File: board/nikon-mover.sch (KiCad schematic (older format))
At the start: 18 parts, among them IC1 ATMEGA8-P, J1 USB, P1 CONN_5, P2 CONN_5, P3 CONN_1, P4 CONN_1, U1 ULN2803, X1 16MHz

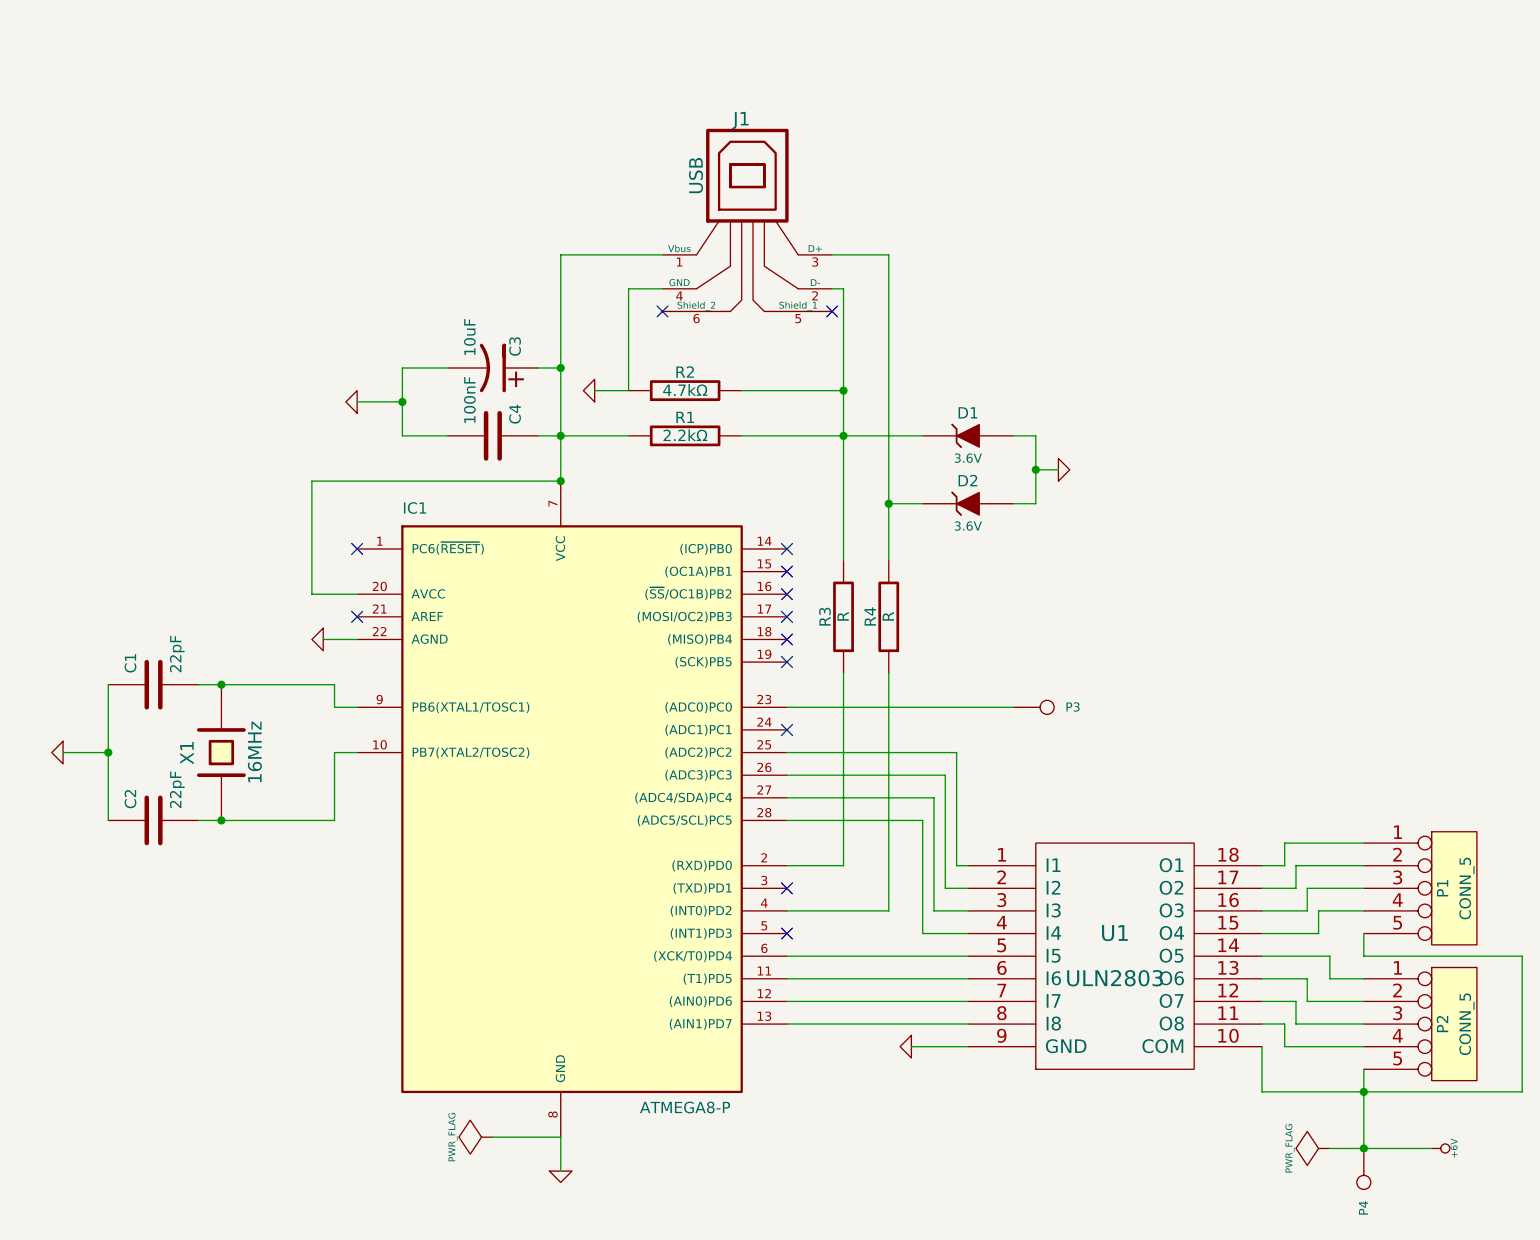
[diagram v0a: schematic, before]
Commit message: Board design
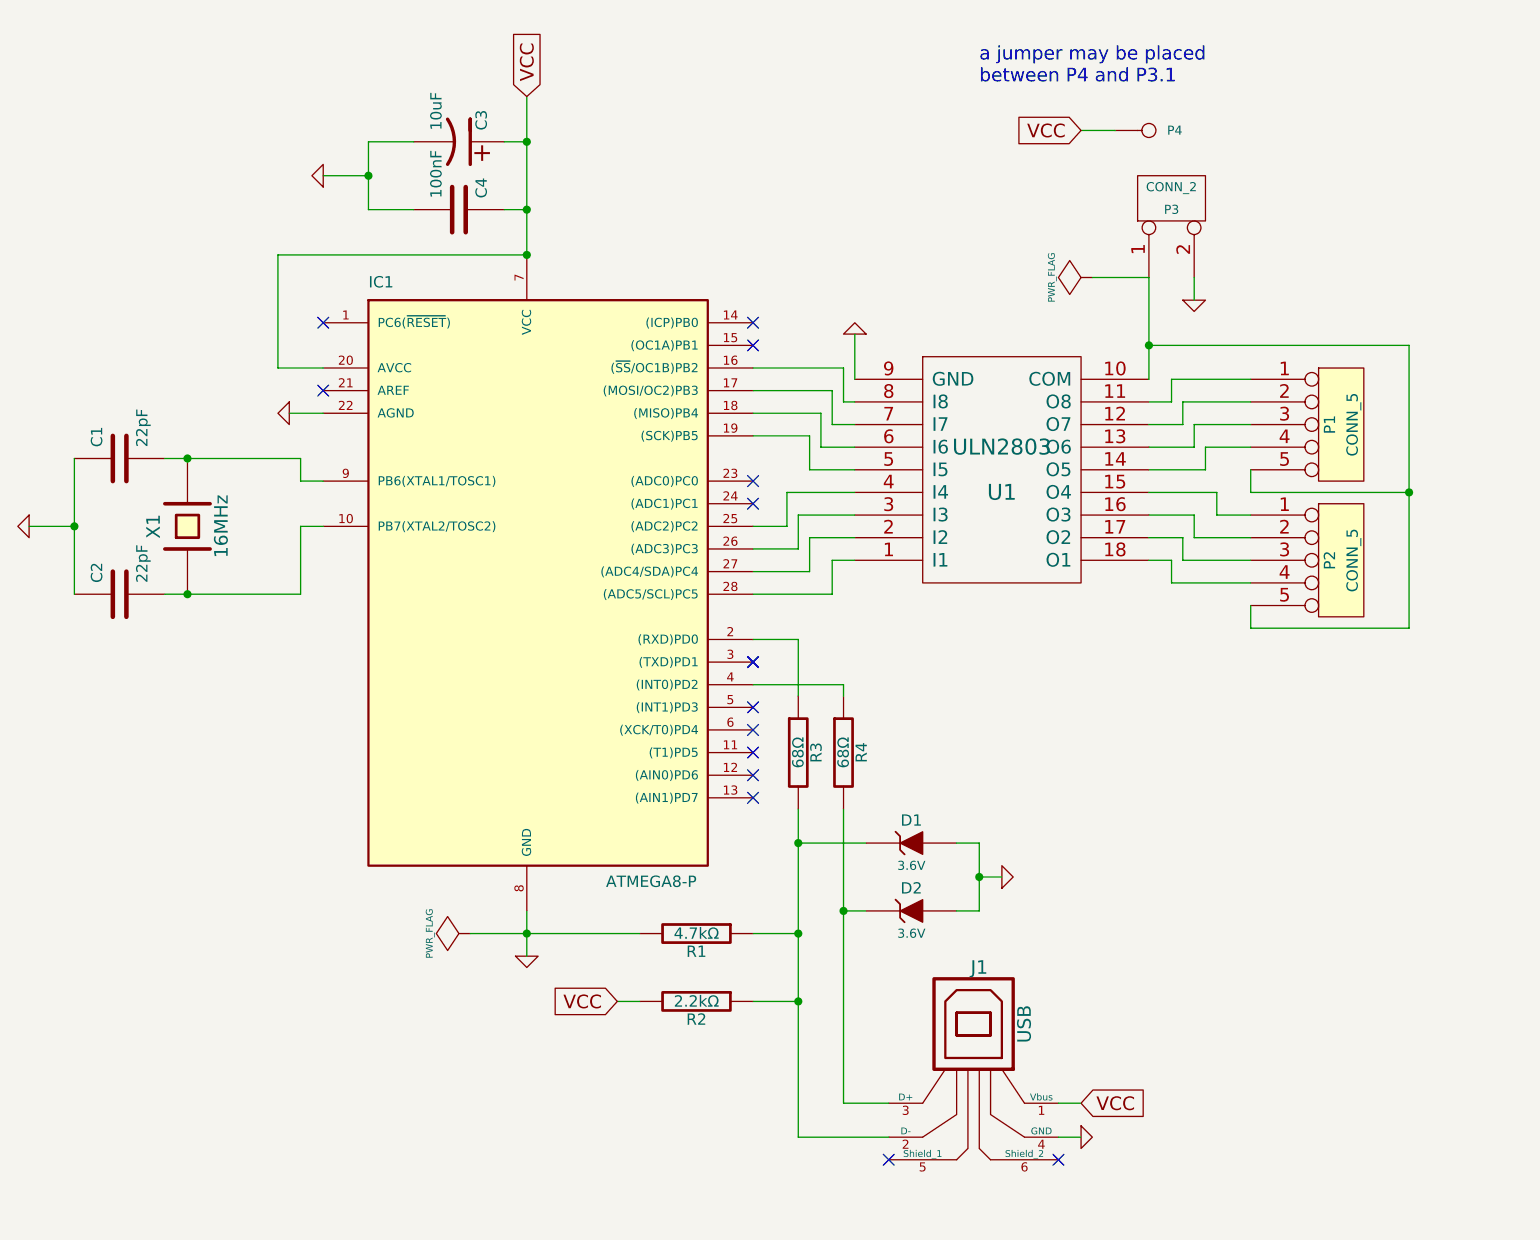
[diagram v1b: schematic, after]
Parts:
- removed P3: CONN_1, symbol CONN_1
- added P3: CONN_2, symbol CONN_2
- R3, R4: value R -> 68Ω
- renumbered R2 to R1, R1 to R2
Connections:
- net GND: now also R1.2, P3.2 (PM); no longer R1.1
- net at IC1.11 ((T1)PD5): no longer U1.6 (I6)
- net at IC1.12 ((AIN0)PD6): no longer U1.7 (I7)
- net at IC1.13 ((AIN1)PD7): no longer U1.8 (I8)
- net at IC1.16 ((~SS~/OC1B)PB2): now also U1.8 (I8)
- net at IC1.17 ((MOSI/OC2)PB3): now also U1.7 (I7)
- net at IC1.18 ((MISO)PB4): now also U1.6 (I6)
- net at IC1.19 ((SCK)PB5): now also U1.5 (I5)
- net VCC: now reaches C3.1, C4.1, IC1.20 (AVCC), IC1.7 (VCC), J1.1 (Vbus)
- net VCC: now also P4.1, R2.2; no longer R2.1
- net at IC1.25 ((ADC2)PC2): now also U1.4 (I4); no longer U1.1 (I1)
- net at IC1.26 ((ADC3)PC3): now also U1.3 (I3); no longer U1.2 (I2)
- net at IC1.27 ((ADC4/SDA)PC4): now also U1.2 (I2); no longer U1.3 (I3)
- net at IC1.28 ((ADC5/SCL)PC5): now also U1.1 (I1); no longer U1.4 (I4)
- net at IC1.6 ((XCK/T0)PD4): no longer U1.5 (I5)
- net at D1.2 (K), J1.2 (D-), R3.2: now also R1.1, R2.1; no longer R1.2, R2.2
- net at U1.11 (O8): now also P1.1; no longer P2.4
- net at U1.12 (O7): now also P1.2; no longer P2.3
- net at U1.13 (O6): now also P1.3; no longer P2.2
- net at U1.14 (O5): now also P1.4; no longer P2.1
- net at U1.15 (O4): now also P2.1; no longer P1.4
- net at U1.16 (O3): now also P2.2; no longer P1.3
- net at U1.17 (O2): now also P2.3; no longer P1.2
- net at U1.18 (O1): now also P2.4; no longer P1.1
- net +6V: no longer names the net of P1.5, P2.5, U1.10 (COM)
- net +6V: now also P3.1 (P1); no longer P4.1
- no-connect marks 13 -> 15
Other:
- note added: "a jumper may be placed\nbetween P4 and P3.1"
- moved on the sheet: C1, C2, C3, C4, D1, D2, IC1, J1, P1, P2, R1, R2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
